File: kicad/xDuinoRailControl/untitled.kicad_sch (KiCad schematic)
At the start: 1 part, among them J1 Barrel_Jack_Switch

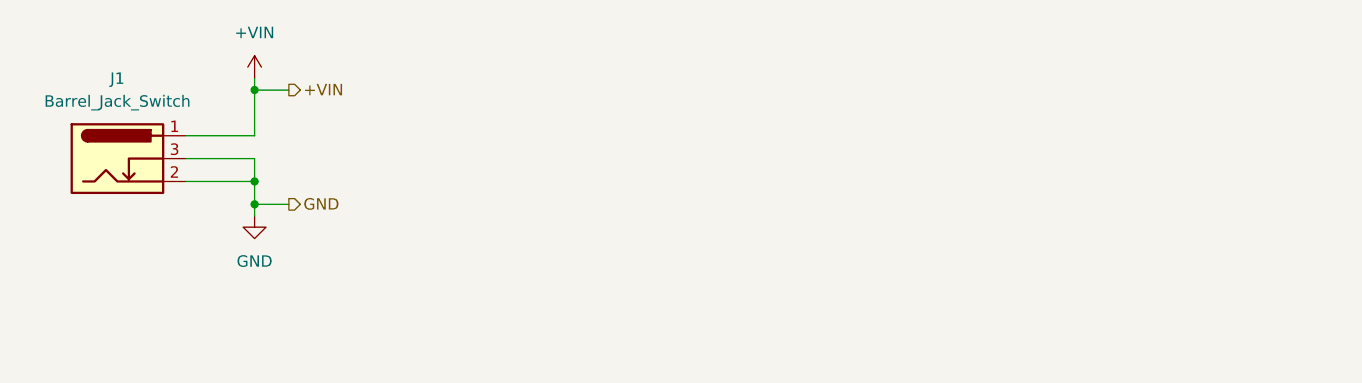
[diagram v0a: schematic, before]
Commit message: xDuinoRailControl
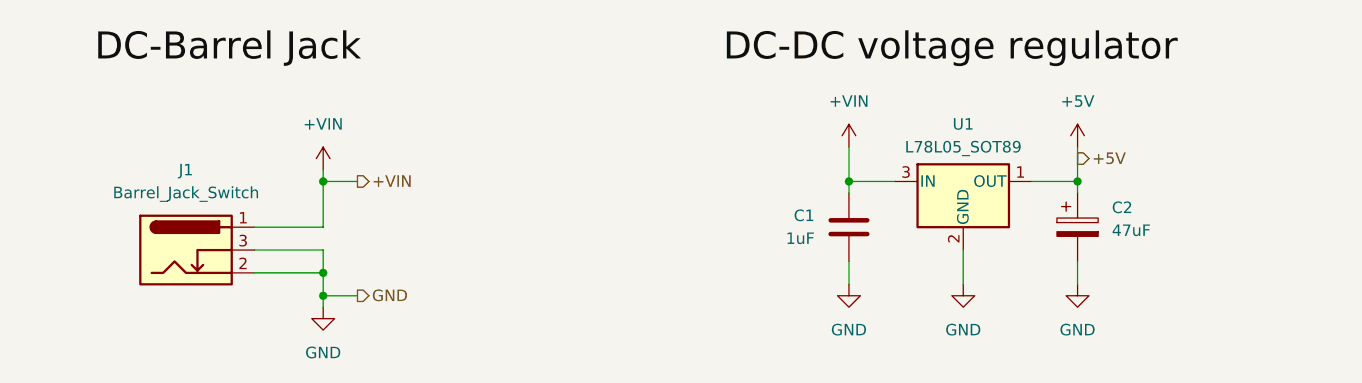
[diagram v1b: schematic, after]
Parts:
- added C1: 1uF, Capacitor_SMD:C_0805_2012Metric_Pad1.18x1.45mm_HandSolder, symbol Device:C
- added C2: 47uF, Capacitor_SMD:C_0805_2012Metric_Pad1.18x1.45mm_HandSolder, symbol Device:C_Polarized
- added U1: L78L05_SOT89, Package_TO_SOT_SMD:SOT-89-3, symbol Regulator_Linear:L78L05_SOT89
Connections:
- net +VIN: now also C1.1, U1.3 (IN)
- net GND: now also C1.2, C2.2, U1.2 (GND)
- new net +5V: C2.1, U1.1 (OUT)
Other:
- moved on the sheet: J1
